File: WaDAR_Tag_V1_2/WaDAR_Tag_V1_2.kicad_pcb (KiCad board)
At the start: 2 copper layers, 34.8 x 41.9 mm, 10 parts, among them J1 SMA-J-P-H-RA-TH1, U1 SIT1534AI-H4-DCC-00.001E

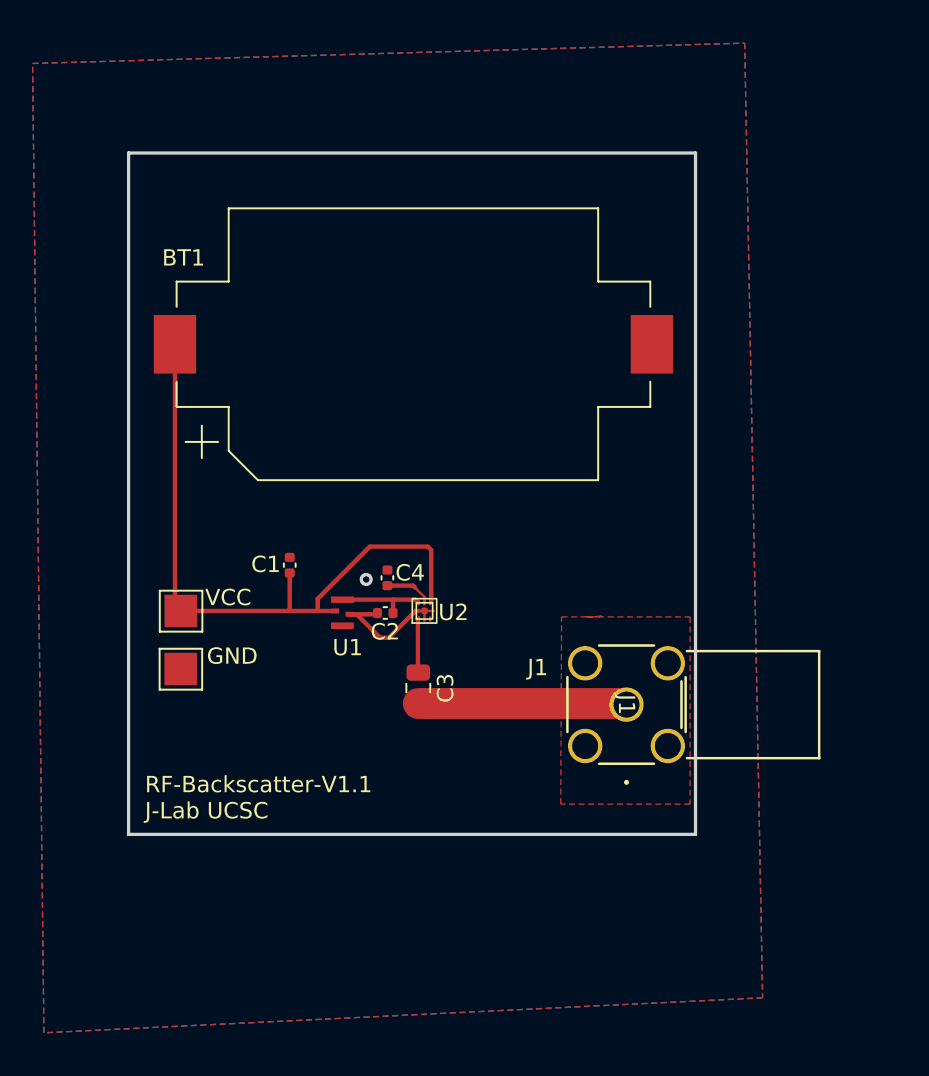
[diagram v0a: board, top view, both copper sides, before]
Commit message: PCB
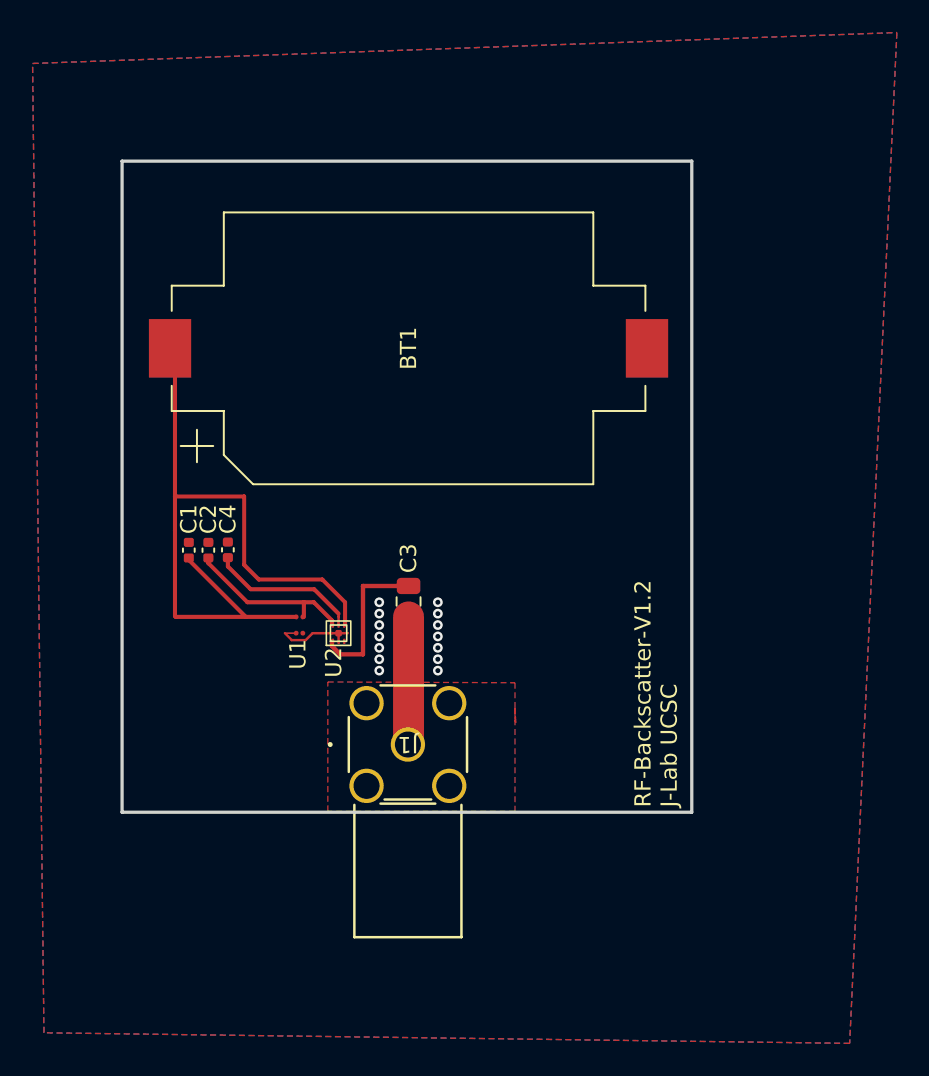
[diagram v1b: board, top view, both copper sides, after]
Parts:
- removed TP1: VCC, JLab_FP:EpicTestPointV1
- removed TP5: GND, JLab_FP:EpicTestPointV1
- U1: value SIT1534AI-H4-DCC-00.001E -> SiT1569; footprint WADARfootprints:XTAL4_SiT1533_SIT -> Library:SiT1569
- moved J1 13.7 mm to (163.6, 81.3), turned to 180 degrees
- moved C2 11.5 mm to (151.3, 69.4), turned to 90 degrees
- moved C4 9.95 mm to (152.5, 69.4)
- moved C1 6.27 mm to (150.1, 69.4)
- moved U2 5.45 mm to (154.6, 74.5)
- moved C3 5.35 mm to (163.6, 72.5)
- moved U1 2.75 mm to (156.9, 74.0)
- moved BT1 0.39 mm to (163.6, 57.0)
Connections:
- U1 pad 2: GND -> Net-(U1-CLK_Out)
- U1 pad 3: Net-(U1-CLK_Out) -> Net-(BT1-+)
- U1 pad 4: Net-(BT1-+) -> GND
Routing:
- net Net-(U2-OUTPUT1): track 3.30 -> 9.67 mm
- net Net-(U2-INPUT): track 2.92 -> 9.24 mm
- net Net-(BT1-+): track 40.7 -> 46.2 mm
- net Net-(U1-CLK_Out): track 5.53 -> 10.6 mm
- net Net-(C3-Pad2): track 12.8 -> 7.86 mm
- net GND: track 7.26 -> 4.00 mm, vias 1 -> 14
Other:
- board size 34.8 x 41.9 mm -> 35 x 40 mm
- board text added: "RF-Backscatter-V1.2 J-Lab UCSC"
- board text removed: "GND"
- board text removed: "J1"
- board text removed: "RF-Backscatter-V1.1 J-Lab UCSC"
- board text removed: "VCC"
